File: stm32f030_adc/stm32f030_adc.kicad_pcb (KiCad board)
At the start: 2 copper layers, 47 parts, among them Q1 BC337, U1 STM32F103C6Tx, U2 AMS1117-3.3, X1 USB_B_Micro, Y2 8 MHz

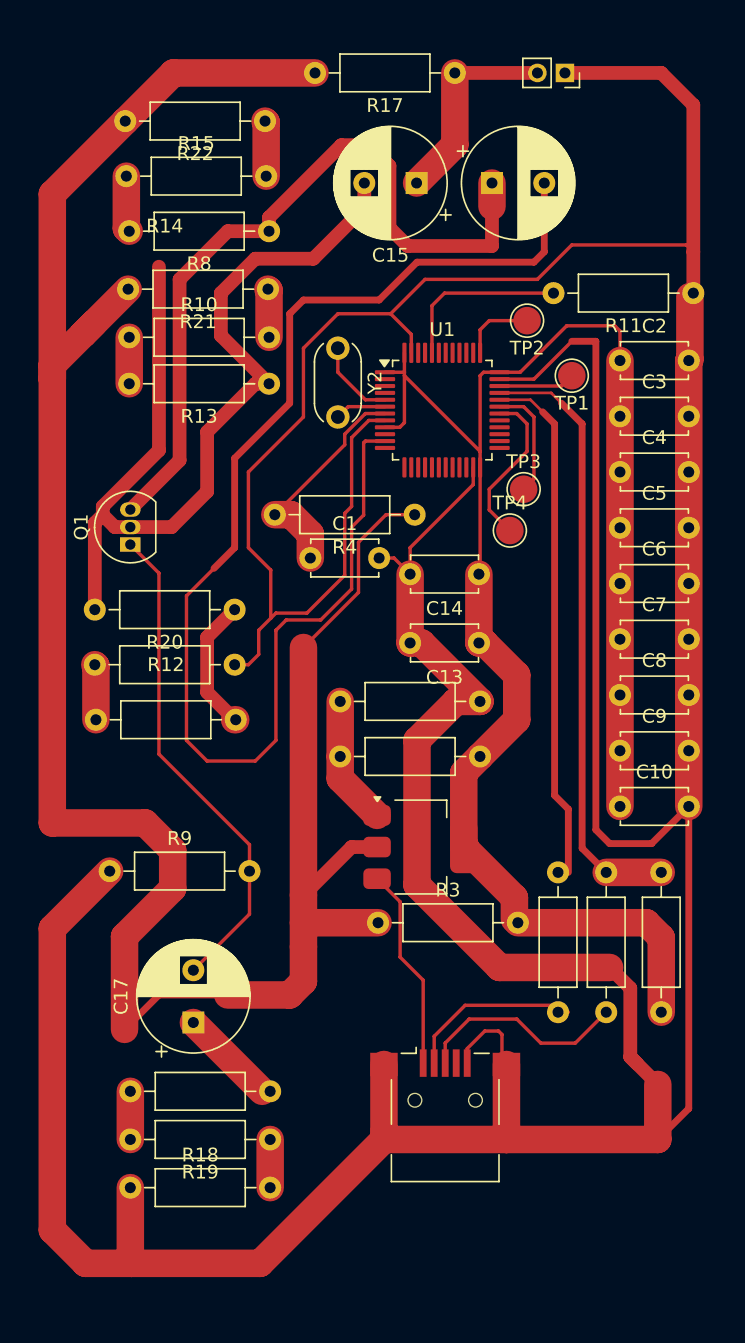
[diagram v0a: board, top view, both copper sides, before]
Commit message: Ref: dead line
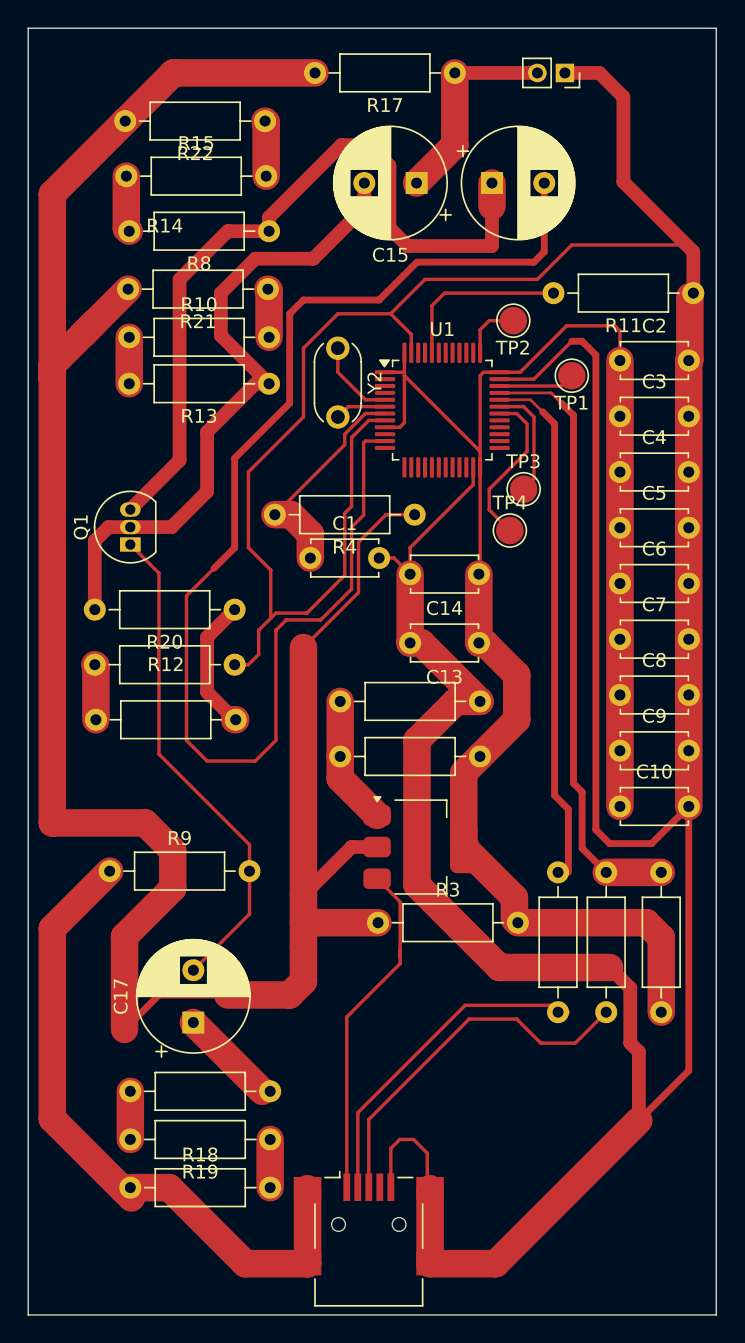
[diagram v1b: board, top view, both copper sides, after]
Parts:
- moved X1 10.6 mm to (148.2, 151.7)
- moved TP2 1.00 mm to (158.8, 86.0)
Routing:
- net GNDREF: track 393.3 -> 367.2 mm
- net Net-(Q1-B): track 69.0 -> 47.8 mm
- net Net-(X1-D+): track 15.5 -> 26.9 mm
- net Net-(X1-D-): track 12.8 -> 24.2 mm
- net 5V_USB: track 14.8 -> 25.2 mm
- net /Power and MCU/SWD_CLK: track 5.36 -> 4.36 mm
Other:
- board outline added: 50 x 93.5 mm
